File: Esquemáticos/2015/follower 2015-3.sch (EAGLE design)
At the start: 16 parts, among them IC1 L293D, X1 TSW-103-02-S-S-RA, X2 TSW-111-02-S-S

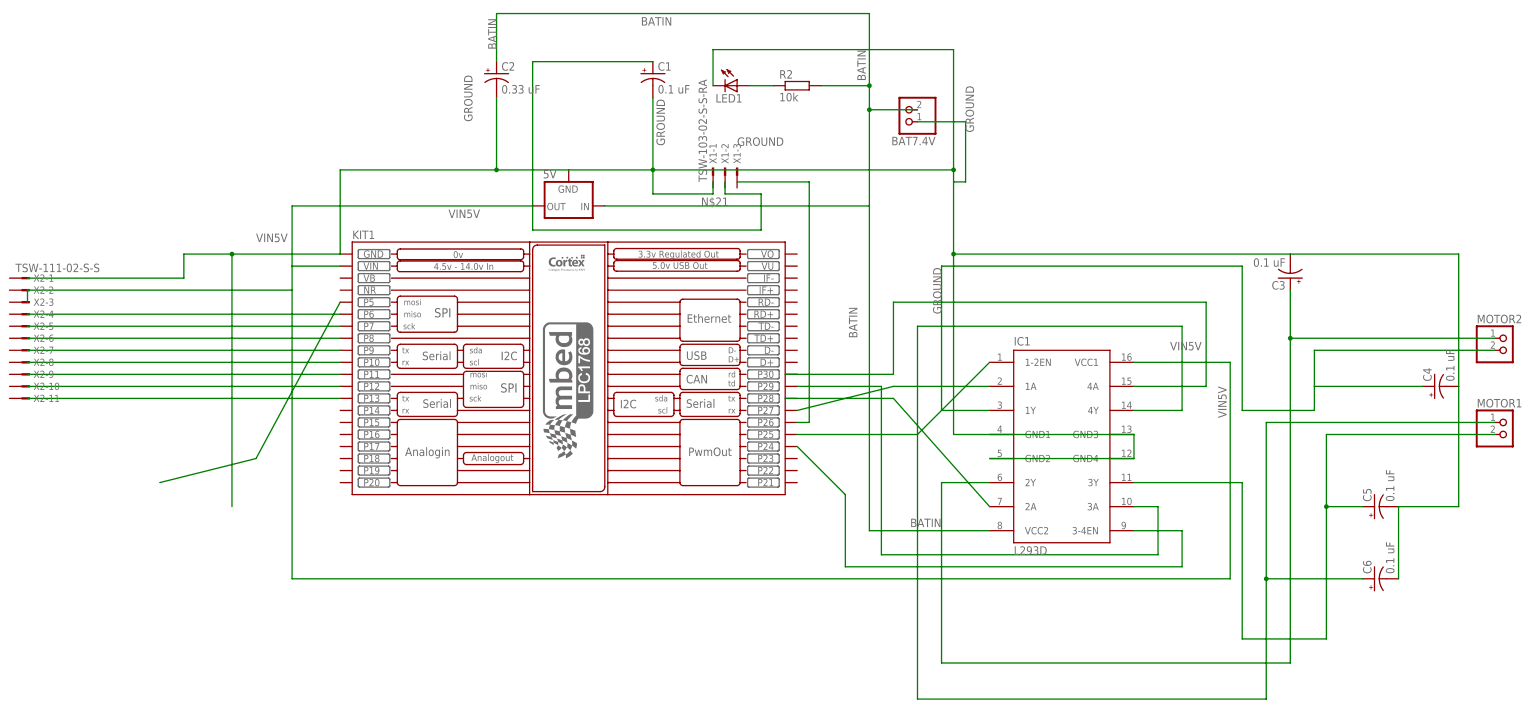
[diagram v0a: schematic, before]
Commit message: Esquemático montado, brincar com a board
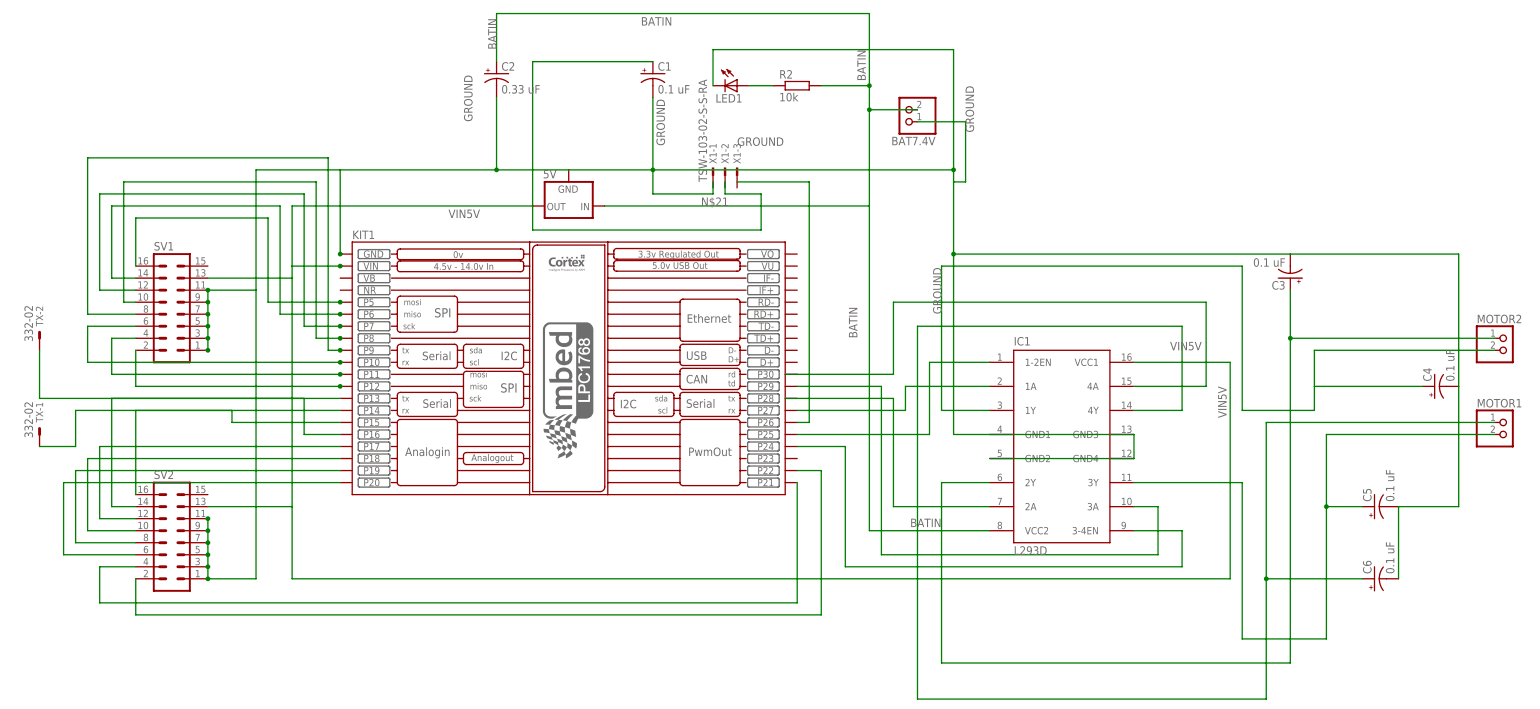
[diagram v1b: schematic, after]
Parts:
- removed X2: TSW-111-02-S-S, con-samtec:TSW-111-02-S-S
- added SV1, SV2: (no value), con-lstb:MA08-2
- added TX: 332-02, con-garry:332-02
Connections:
- new net N$20: KIT1.P16, SV2.14
- new net N$23: KIT1.P17, SV2.12
- new net N$24: KIT1.P18, SV2.10
- new net N$25: KIT1.P19, SV2.8
- new net N$26: KIT1.P20, SV2.6
- new net N$27: KIT1.P21, SV2.4
- new net N$28: KIT1.P22, SV2.2
- new net RX: KIT1.P14, TX-1.S
- new net TX: KIT1.P13, TX-2.S
- net GROUND: now also SV1.1, SV1.11, SV1.3, SV1.5, SV1.7, SV1.9, SV2.1, SV2.11, SV2.3, SV2.5, SV2.7, SV2.9
- net N$1: now also KIT1.P11, SV1.4; no longer KIT1.P5
- net N$11: now also KIT1.P5, SV1.16; no longer KIT1.P6
- net N$12: now also KIT1.P6, SV1.14; no longer KIT1.P7
- net N$13: now also KIT1.P7, SV1.12; no longer KIT1.P8
- net N$14: now also KIT1.P8, SV1.10; no longer KIT1.P9
- net N$15: now also KIT1.P9, SV1.8; no longer KIT1.P10
- net N$16: now also KIT1.P10, SV1.6; no longer KIT1.P11
- net N$17: now also SV1.2
- net N$18: now also KIT1.P15, SV2.16; no longer KIT1.P13
- net VIN5V: now also SV1.13, SV2.13
